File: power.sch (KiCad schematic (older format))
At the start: 22 parts, among them J4 USB_C_Receptacle_USB2.0, Q10 Q_PMOS_GDS, SW1 SW_SPST, U13 TP4056, U14 TPS63001DRCR

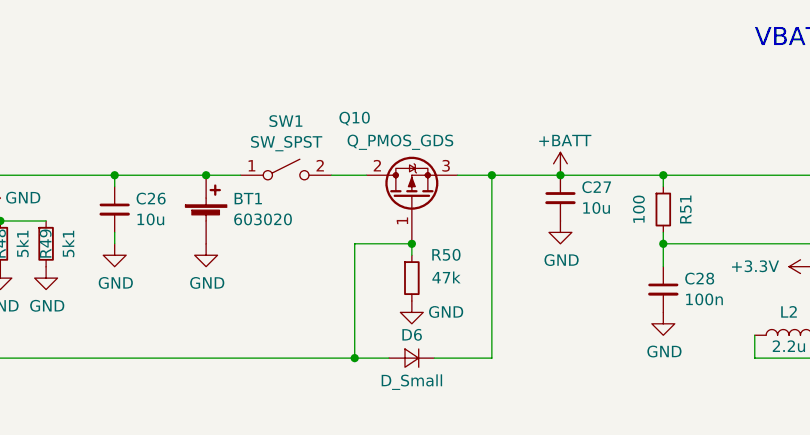
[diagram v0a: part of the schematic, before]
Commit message: ADD:started to place footprints
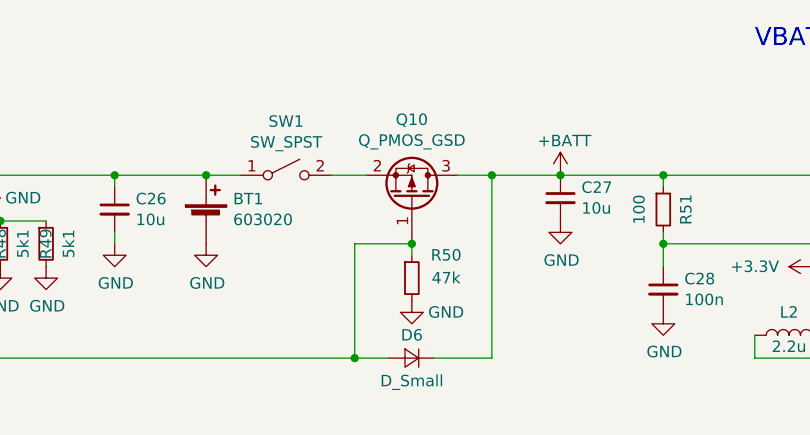
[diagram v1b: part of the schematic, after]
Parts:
- removed Q10: Q_PMOS_GDS, Package_TO_SOT_SMD:SOT-23, symbol Device:Q_PMOS_GDS
- added Q10: Q_PMOS_GSD, symbol Device:Q_PMOS_GSD
- C24, C28, C29: footprint Capacitor_SMD:C_0603_1608Metric -> Capacitor_SMD:C_0402_1005Metric
- D6: footprint Diode_SMD:D_SMA -> Diode_SMD:D_SOD-123F
- R45, R46, R47, R48, R49, R50, R51: footprint Resistor_SMD:R_0603_1608Metric -> Resistor_SMD:R_0402_1005Metric
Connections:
- net +BATT: now also Q10.3 (D)
- net VBUS: now also Q10.1 (G)
- net at SW1.2 (B): now also Q10.2 (S)
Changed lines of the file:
@@
 F 0 "R45" V 2400 2950 50  0000 C CNN
 F 1 "5k1" V 2295 2950 50  0000 C CNN
-F 2 "Resistor_SMD:R_0603_1608Metric" H 2400 2950 50  0001 C CNN
+F 2 "Resistor_SMD:R_0402_1005Metric" H 2400 2950 50  0001 C CNN
 F 3 "~" H 2400 2950 50  0001 C CNN
 	1    2400 2950
@@
 F 0 "R46" V 2400 3050 50  0000 C CNN
 F 1 "5k1" V 2500 3050 50  0000 C CNN
-F 2 "Resistor_SMD:R_0603_1608Metric" H 2400 3050 50  0001 C CNN
+F 2 "Resistor_SMD:R_0402_1005Metric" H 2400 3050 50  0001 C CNN
 F 3 "~" H 2400 3050 50  0001 C CNN
 	1    2400 3050
@@
 F 0 "C24" V 1550 3950 50  0000 L CNN
 F 1 "100p" V 1550 4100 50  0000 L CNN
-F 2 "Capacitor_SMD:C_0603_1608Metric" H 1400 4250 50  0001 C CNN
+F 2 "Capacitor_SMD:C_0402_1005Metric" H 1400 4250 50  0001 C CNN
 F 3 "~" H 1400 4250 50  0001 C CNN
 	1    1400 4250
@@
 F 0 "C28" H 7592 3296 50  0000 L CNN
 F 1 "100n" H 7592 3205 50  0000 L CNN
-F 2 "Capacitor_SMD:C_0603_1608Metric" H 7500 3250 50  0001 C CNN
+F 2 "Capacitor_SMD:C_0402_1005Metric" H 7500 3250 50  0001 C CNN
 F 3 "~" H 7500 3250 50  0001 C CNN
 	1    7500 3250
@@
 F 0 "R51" V 7600 2900 50  0000 C CNN
 F 1 "100" V 7395 2900 50  0000 C CNN
-F 2 "Resistor_SMD:R_0603_1608Metric" H 7500 2900 50  0001 C CNN
+F 2 "Resistor_SMD:R_0402_1005Metric" H 7500 2900 50  0001 C CNN
 F 3 "~" H 7500 2900 50  0001 C CNN
 	1    7500 2900
@@
 F 0 "C29" H 10042 2896 50  0000 L CNN
 F 1 "100n" H 10042 2805 50  0000 L CNN
-F 2 "Capacitor_SMD:C_0603_1608Metric" H 9950 2850 50  0001 C CNN
+F 2 "Capacitor_SMD:C_0402_1005Metric" H 9950 2850 50  0001 C CNN
 F 3 "~" H 9950 2850 50  0001 C CNN
 	1    9950 2850
@@
 F 0 "R47" V 3096 3650 50  0000 C CNN
 F 1 "390k" V 3005 3650 50  0000 C CNN
-F 2 "Resistor_SMD:R_0603_1608Metric" H 2900 3650 50  0001 C CNN
+F 2 "Resistor_SMD:R_0402_1005Metric" H 2900 3650 50  0001 C CNN
 F 3 "~" H 2900 3650 50  0001 C CNN
 	1    2900 3650
@@
 $EndComp
 Connection ~ 5100 2750
-$Comp
-L Device:Q_PMOS_GDS Q10
-U 1 1 5CBC71E1
-P 6400 2850
-F 0 "Q10" V 6750 3100 50  0000 C CNN
-F 1 "Q_PMOS_GDS" V 6650 2900 50  0000 C CNN
-F 2 "Package_TO_SOT_SMD:SOT-23" H 6600 2950 50  0001 C CNN
-F 3 "~" H 6400 2850 50  0001 C CNN
-	1    6400 2850
-	0    -1   -1   0
-$EndComp
 Wire Wire Line
 	5100 2800 5100 2750
@@
 F 0 "R50" H 6550 3300 50  0000 C CNN
 F 1 "47k" H 6550 3200 50  0000 C CNN
-F 2 "Resistor_SMD:R_0603_1608Metric" H 6400 3200 50  0001 C CNN
+F 2 "Resistor_SMD:R_0402_1005Metric" H 6400 3200 50  0001 C CNN
 F 3 "~" H 6400 3200 50  0001 C CNN
 	1    6400 3200
@@
 Wire Wire Line
 	6400 3100 6400 3050
-Connection ~ 6400 3050
 $Comp
 L Device:D_Small D6
@@
 F 0 "D6" H 6400 3450 50  0000 C CNN
 F 1 "D_Small" H 6400 3650 50  0000 C CNN
-F 2 "Diode_SMD:D_SMA" V 6400 3550 50  0001 C CNN
+F 2 "Diode_SMD:D_SOD-123F" V 6400 3550 50  0001 C CNN
 F 3 "~" V 6400 3550 50  0001 C CNN
 	1    6400 3550
@@
 F 0 "R48" V 4600 3050 50  0000 C CNN
 F 1 "5k1" V 4700 3050 50  0000 C CNN
-F 2 "Resistor_SMD:R_0603_1608Metric" H 4600 3050 50  0001 C CNN
+F 2 "Resistor_SMD:R_0402_1005Metric" H 4600 3050 50  0001 C CNN
 F 3 "~" H 4600 3050 50  0001 C CNN
 	1    4600 3050
@@
 F 0 "R49" V 4800 3050 50  0000 C CNN
 F 1 "5k1" V 4900 3050 50  0000 C CNN
-F 2 "Resistor_SMD:R_0603_1608Metric" H 4800 3050 50  0001 C CNN
+F 2 "Resistor_SMD:R_0402_1005Metric" H 4800 3050 50  0001 C CNN
 F 3 "~" H 4800 3050 50  0001 C CNN
 	1    4800 3050
@@
 	5650 2750 5500 2750
 Connection ~ 5500 2750
+$Comp
+L Device:Q_PMOS_GSD Q?
+U 1 1 5CE12F3D
+P 6400 2850
+AR Path="/5CE12F3D" Ref="Q?"  Part="1"
+AR Path="/5C753B69/5CE12F3D" Ref="Q10"  Part="1"
+F 0 "Q10" V 6743 2850 50  0000 C CNN
+F 1 "Q_PMOS_GSD" V 6652 2850 50  0000 C CNN
+F 2 "" H 6600 2950 50  0001 C CNN
+F 3 "~" H 6400 2850 50  0001 C CNN
+	1    6400 2850
+	0    1    -1   0
+$EndComp
+Connection ~ 6400 3050
 $EndSCHEMATC

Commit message: ADD: started routing
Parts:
- Q10: footprint (none) -> Package_TO_SOT_SMD:SOT-23
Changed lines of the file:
@@
 F 0 "Q10" V 6743 2850 50  0000 C CNN
 F 1 "Q_PMOS_GSD" V 6652 2850 50  0000 C CNN
-F 2 "" H 6600 2950 50  0001 C CNN
+F 2 "Package_TO_SOT_SMD:SOT-23" H 6600 2950 50  0001 C CNN
 F 3 "~" H 6400 2850 50  0001 C CNN
 	1    6400 2850
